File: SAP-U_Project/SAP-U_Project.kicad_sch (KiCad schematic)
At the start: 0 parts

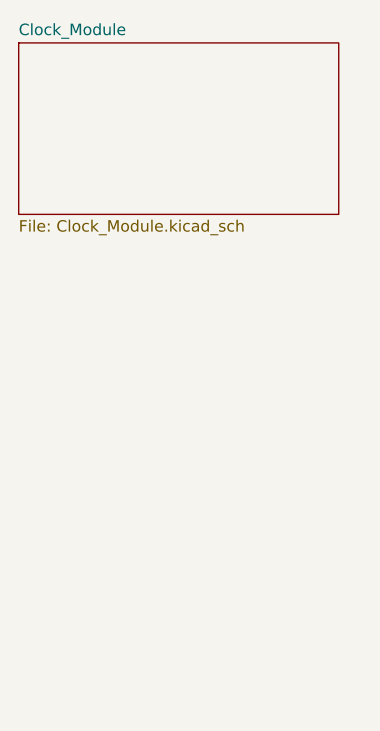
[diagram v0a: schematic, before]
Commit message: Checkpoint: completed schematic for Clock Module
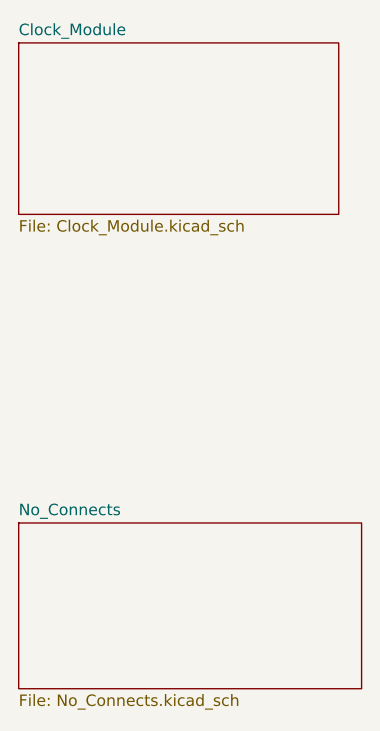
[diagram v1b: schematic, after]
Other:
- added sheet No_Connects (No_Connects.kicad_sch)
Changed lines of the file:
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@@
+		)
+	)
+	(sheet
+		(at 30.48 82.55)
+		(size 38.1 18.415)
+		(fields_autoplaced yes)
+		(stroke
+			(width 0.1524)
+			(type solid)
+		)
+		(fill
+			(color 0 0 0 0.0000)
+		)
+		(property "Sheetname" "No_Connects"
+			(at 30.48 81.8384 0)
+			(effects
+				(font
+					(size 1.27 1.27)
+				)
+				(justify left bottom)
+			)
+		)
+		(property "Sheetfile" "No_Connects.kicad_sch"
+			(at 30.48 101.5496 0)
+			(effects
+				(font
+					(size 1.27 1.27)
+				)
+				(justify left top)
+			)
+		)
+		(instances
+			(project "SAP-U_Project"
+				(path "/e63e39d7-6ac0-4ffd-8aa3-1841a4541b55"
+					(page "3")
+				)
+			)
 		)
 	)
